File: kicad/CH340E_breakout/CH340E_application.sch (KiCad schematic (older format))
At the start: 10 parts, among them U2 HT42B534-MSOP10

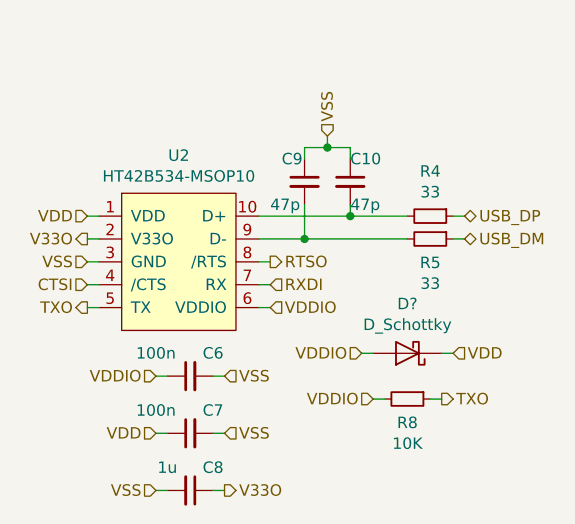
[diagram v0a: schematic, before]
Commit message: schematic and routing completed
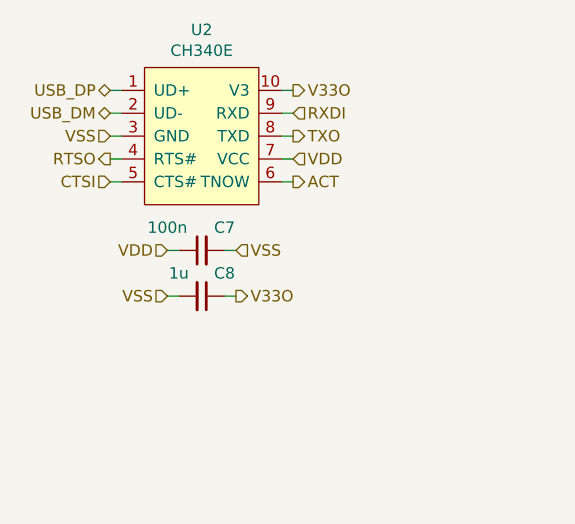
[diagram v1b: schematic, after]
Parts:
- removed C10, C9: 47p, SquantorRcl:C_0402, symbol Device:C_Small
- removed C6: 100n, SquantorRcl:C_0402, symbol Device:C_Small
- removed D?: D_Schottky, SquantorDiodes:SOD-523, symbol Device:D_Schottky
- removed R4, R5: 33, SquantorRcl:R_0402_hand, symbol Device:R_Small
- removed R8: 10K, SquantorRcl:R_0402_hand, symbol Device:R_Small
- removed U2: HT42B534-MSOP10, SquantorIC:MSOP-10, symbol SquantorHoltek:HT42B534-MSOP10
- added U2: CH340E, SquantorIC:MSOP-10, symbol SquantorWCH:CH340E
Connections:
- net CTSI: now also U2.5 (CTS#)
- net RTSO: now also U2.4 (RTS#)
- net RXDI: now also U2.9 (RXD)
- net TXO: now also U2.8 (TXD)
- net USB_DM: now also U2.2 (UD-)
- net USB_DP: now also U2.1 (UD+)
- net V33O: now also U2.10 (V3)
- net VDD: now also U2.7 (VCC)
- net VSS: now also U2.3 (GND)
- new net ACT: U2.6 (TNOW)
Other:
- moved on the sheet: C7, C8
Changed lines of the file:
@@
 Comment4 ""
 $EndDescr
-Wire Wire Line
-	3500 2000 3750 2000
-Wire Wire Line
-	3500 1950 3500 2000
-Wire Wire Line
-	3300 2100 3750 2100
-Wire Wire Line
-	3300 1950 3300 2100
-Wire Wire Line
-	3500 1700 3400 1700
-Wire Wire Line
-	3500 1750 3500 1700
-Wire Wire Line
-	3400 1700 3400 1650
-Connection ~ 3400 1700
-Wire Wire Line
-	3300 1700 3400 1700
-Wire Wire Line
-	3300 1750 3300 1700
-$Comp
-L Device:C_Small C?
-U 1 1 5C9D5468
-P 3300 1850
-AR Path="/5C9D5468" Ref="C?"  Part="1"
-AR Path="/5C9B7479/5C9D5468" Ref="C9"  Part="1"
-F 0 "C9" H 3200 1950 50  0000 L CNN
-F 1 "47p" H 3150 1750 50  0000 L CNN
-F 2 "SquantorRcl:C_0402" H 3300 1850 50  0001 C CNN
-F 3 "~" H 3300 1850 50  0001 C CNN
-	1    3300 1850
-	1    0    0    -1
-$EndComp
-$Comp
-L Device:C_Small C?
-U 1 1 5C9D546E
-P 3500 1850
-AR Path="/5C9D546E" Ref="C?"  Part="1"
-AR Path="/5C9B7479/5C9D546E" Ref="C10"  Part="1"
-F 0 "C10" H 3500 1950 50  0000 L CNN
-F 1 "47p" H 3500 1750 50  0000 L CNN
-F 2 "SquantorRcl:C_0402" H 3500 1850 50  0001 C CNN
-F 3 "~" H 3500 1850 50  0001 C CNN
-	1    3500 1850
-	1    0    0    -1
-$EndComp
-Wire Wire Line
-	3950 2000 4000 2000
-Connection ~ 3500 2000
-Wire Wire Line
-	3100 2000 3500 2000
-Connection ~ 3300 2100
-Wire Wire Line
-	3100 2100 3300 2100
-Wire Wire Line
-	4000 2100 3950 2100
-$Comp
-L Device:R_Small R?
-U 1 1 5C9D547C
-P 3850 2100
-AR Path="/5C9D547C" Ref="R?"  Part="1"
-AR Path="/5C9B7479/5C9D547C" Ref="R5"  Part="1"
-F 0 "R5" V 3954 2100 50  0000 C CNN
-F 1 "33" V 4045 2100 50  0000 C CNN
-F 2 "SquantorRcl:R_0402_hand" H 3850 2100 50  0001 C CNN
-F 3 "~" H 3850 2100 50  0001 C CNN
-	1    3850 2100
-	0    1    1    0
-$EndComp
-$Comp
-L Device:R_Small R?
-U 1 1 5C9D5482
-P 3850 2000
-AR Path="/5C9D5482" Ref="R?"  Part="1"
-AR Path="/5C9B7479/5C9D5482" Ref="R4"  Part="1"
-F 0 "R4" V 3654 2000 50  0000 C CNN
-F 1 "33" V 3745 2000 50  0000 C CNN
-F 2 "SquantorRcl:R_0402_hand" H 3850 2000 50  0001 C CNN
-F 3 "~" H 3850 2000 50  0001 C CNN
-	1    3850 2000
-	0    1    1    0
-$EndComp
-Wire Wire Line
-	3100 2300 3150 2300
-Wire Wire Line
-	3100 2200 3150 2200
-Wire Wire Line
-	2700 2700 2650 2700
-Wire Wire Line
-	2900 2700 2950 2700
-$Comp
-L Device:C_Small C?
-U 1 1 5C9D548C
-P 2800 2700
-AR Path="/5C9D548C" Ref="C?"  Part="1"
-AR Path="/5C9B7479/5C9D548C" Ref="C6"  Part="1"
-F 0 "C6" V 2900 2600 50  0000 C CNN
-F 1 "100n" V 2900 2850 50  0000 C CNN
-F 2 "SquantorRcl:C_0402" H 2800 2700 50  0001 C CNN
-F 3 "~" H 2800 2700 50  0001 C CNN
-	1    2800 2700
-	0    -1   -1   0
-$EndComp
-Wire Wire Line
-	3100 2400 3150 2400
-Wire Wire Line
-	2400 2400 2350 2400
-Wire Wire Line
-	2400 2300 2350 2300
-Wire Wire Line
-	2350 2000 2400 2000
-$Comp
-L SquantorHoltek:HT42B534-MSOP10 U?
-U 1 1 5C9D54C0
-P 2750 2200
-AR Path="/5C9D54C0" Ref="U?"  Part="1"
-AR Path="/5C9B7479/5C9D54C0" Ref="U2"  Part="1"
-F 0 "U2" H 2750 2665 50  0000 C CNN
-F 1 "HT42B534-MSOP10" H 2750 2574 50  0000 C CNN
-F 2 "SquantorIC:MSOP-10" H 2750 2100 50  0001 C CNN
-F 3 "" H 2750 2100 50  0001 C CNN
-	1    2750 2200
-	1    0    0    -1
-$EndComp
-Text HLabel 2350 2200 0    50   Input ~ 0
+Text HLabel 3000 2150 2    50   Input ~ 0
 VSS
-Text HLabel 2350 2000 0    50   Input ~ 0
-VDD
-Text HLabel 3400 1650 1    50   Input ~ 0
-VSS
-Text HLabel 2950 2700 2    50   Input ~ 0
-VSS
-Text HLabel 3150 2400 2    50   Input ~ 0
-VDDIO
-Wire Wire Line
-	2350 2200 2400 2200
-Text HLabel 2350 2100 0    50   Output ~ 0
-V33O
-Wire Wire Line
-	2400 2100 2350 2100
-Text HLabel 2650 2700 0    50   Input ~ 0
-VDDIO
-Text HLabel 4000 2100 2    50   BiDi ~ 0
-USB_DM
-Text HLabel 4000 2000 2    50   BiDi ~ 0
-USB_DP
-Text HLabel 3150 2300 2    50   Input ~ 0
-RXDI
-Text HLabel 3150 2200 2    50   Output ~ 0
-RTSO
-Text HLabel 2350 2400 0    50   Output ~ 0
-TXO
-Text HLabel 2350 2300 0    50   Input ~ 0
-CTSI
-Text HLabel 2950 2950 2    50   Input ~ 0
-VSS
-Text HLabel 2650 2950 0    50   Input ~ 0
+Text HLabel 2700 2150 0    50   Input ~ 0
 VDD
 $Comp
 L Device:C_Small C?
 U 1 1 5C9D549F
-P 2800 2950
+P 2850 2150
 AR Path="/5C9D549F" Ref="C?"  Part="1"
 AR Path="/5C9B7479/5C9D549F" Ref="C7"  Part="1"
-F 0 "C7" V 2900 2850 50  0000 C CNN
-F 1 "100n" V 2900 3100 50  0000 C CNN
-F 2 "SquantorRcl:C_0402" H 2800 2950 50  0001 C CNN
-F 3 "~" H 2800 2950 50  0001 C CNN
-	1    2800 2950
+F 0 "C7" V 2950 2050 50  0000 C CNN
+F 1 "100n" V 2950 2300 50  0000 C CNN
+F 2 "SquantorRcl:C_0402" H 2850 2150 50  0001 C CNN
+F 3 "~" H 2850 2150 50  0001 C CNN
+	1    2850 2150
 	0    -1   -1   0
 $EndComp
 Wire Wire Line
-	2650 2950 2700 2950
+	2700 2150 2750 2150
 Wire Wire Line
-	2900 2950 2950 2950
+	2950 2150 3000 2150
 Wire Wire Line
-	2900 3200 2950 3200
+	2950 2350 3000 2350
 Wire Wire Line
-	2650 3200 2700 3200
-Text HLabel 2950 3200 2    50   Output ~ 0
+	2700 2350 2750 2350
+Text HLabel 3000 2350 2    50   Output ~ 0
 V33O
-Text HLabel 2650 3200 0    50   Input ~ 0
+Text HLabel 2700 2350 0    50   Input ~ 0
 VSS
 $Comp
 L Device:C_Small C?
 U 1 1 5C9D54B3
-P 2800 3200
+P 2850 2350
 AR Path="/5C9D54B3" Ref="C?"  Part="1"
 AR Path="/5C9B7479/5C9D54B3" Ref="C8"  Part="1"
-F 0 "C8" V 2700 3300 50  0000 C CNN
-F 1 "1u" V 2700 3100 50  0000 C CNN
-F 2 "SquantorRcl:C_0603" H 2800 3200 50  0001 C CNN
-F 3 "~" H 2800 3200 50  0001 C CNN
-	1    2800 3200
+F 0 "C8" V 2750 2450 50  0000 C CNN
+F 1 "1u" V 2750 2250 50  0000 C CNN
+F 2 "SquantorRcl:C_0603" H 2850 2350 50  0001 C CNN
+F 3 "~" H 2850 2350 50  0001 C CNN
+	1    2850 2350
 	0    1    1    0
 $EndComp
-Text HLabel 3600 2800 0    50   Input ~ 0
-VDDIO
-$Comp
-L Device:R_Small R?
-U 1 1 5C9AB245
-P 3750 2800
-AR Path="/5C9AB245" Ref="R?"  Part="1"
-AR Path="/5C9B7479/5C9AB245" Ref="R8"  Part="1"
-F 0 "R8" V 3854 2800 50  0000 C CNN
-F 1 "10K" V 3945 2800 50  0000 C CNN
-F 2 "SquantorRcl:R_0402_hand" H 3750 2800 50  0001 C CNN
-F 3 "~" H 3750 2800 50  0001 C CNN
-	1    3750 2800
-	0    1    1    0
-$EndComp
-Text HLabel 3900 2800 2    50   Output ~ 0
+Text HLabel 2450 1550 0    50   BiDi ~ 0
+USB_DM
+Wire Wire Line
+	2450 1550 2500 1550
+Text HLabel 2450 1450 0    50   BiDi ~ 0
+USB_DP
+Wire Wire Line
+	2500 1450 2450 1450
+Text HLabel 3250 1550 2    50   Input ~ 0
+RXDI
+Wire Wire Line
+	3200 1550 3250 1550
+Text HLabel 3250 1650 2    50   Output ~ 0
 TXO
 Wire Wire Line
-	3600 2800 3650 2800
+	3200 1450 3250 1450
+Text HLabel 3250 1450 2    50   Output ~ 0
+V33O
 Wire Wire Line
-	3850 2800 3900 2800
-Text HLabel 3550 2600 0    50   Input ~ 0
-VDDIO
+	2450 1650 2500 1650
+Text HLabel 3250 1750 2    50   Input ~ 0
+VDD
+Text HLabel 2450 1650 0    50   Input ~ 0
+VSS
+Wire Wire Line
+	3250 1750 3200 1750
+Wire Wire Line
+	3200 1650 3250 1650
+Wire Wire Line
+	2500 1850 2450 1850
+Text HLabel 2450 1850 0    50   Input ~ 0
+CTSI
+Wire Wire Line
+	2500 1750 2450 1750
+Text HLabel 2450 1750 0    50   Output ~ 0
+RTSO
 $Comp
-L Device:D_Schottky D?
-U 1 1 5C9D33D2
-P 3750 2600
-F 0 "D?" H 3750 2384 50  0000 C CNN
-F 1 "D_Schottky" H 3750 2475 50  0000 C CNN
-F 2 "SquantorDiodes:SOD-523" H 3750 2600 50  0001 C CNN
-F 3 "~" H 3750 2600 50  0001 C CNN
-	1    3750 2600
-	-1   0    0    1
+L SquantorWCH:CH340E U2
+U 1 1 5CA3A399
+P 2850 1650
+F 0 "U2" H 2850 2115 50  0000 C CNN
+F 1 "CH340E" H 2850 2024 50  0000 C CNN
+F 2 "SquantorIC:MSOP-10" H 2850 1550 50  0001 C CNN
+F 3 "" H 2850 1550 50  0001 C CNN
+	1    2850 1650
+	1    0    0    -1
 $EndComp
+Text HLabel 3250 1850 2    50   Output ~ 0
+ACT
 Wire Wire Line
-	3600 2600 3550 2600
-Text HLabel 3950 2600 2    50   Input ~ 0
-VDD
-Wire Wire Line
-	3950 2600 3900 2600
+	3200 1850 3250 1850
 $EndSCHEMATC
